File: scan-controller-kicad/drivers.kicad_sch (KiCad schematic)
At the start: 45 parts, among them CN4 Fan, CN5 Motor, CN6 Lamp, Q6 SS8050, Q7 IRF7470, U5 DRV8871DDA, U6 78L05, U7 XL4015, U8 TL431, U9 LM358

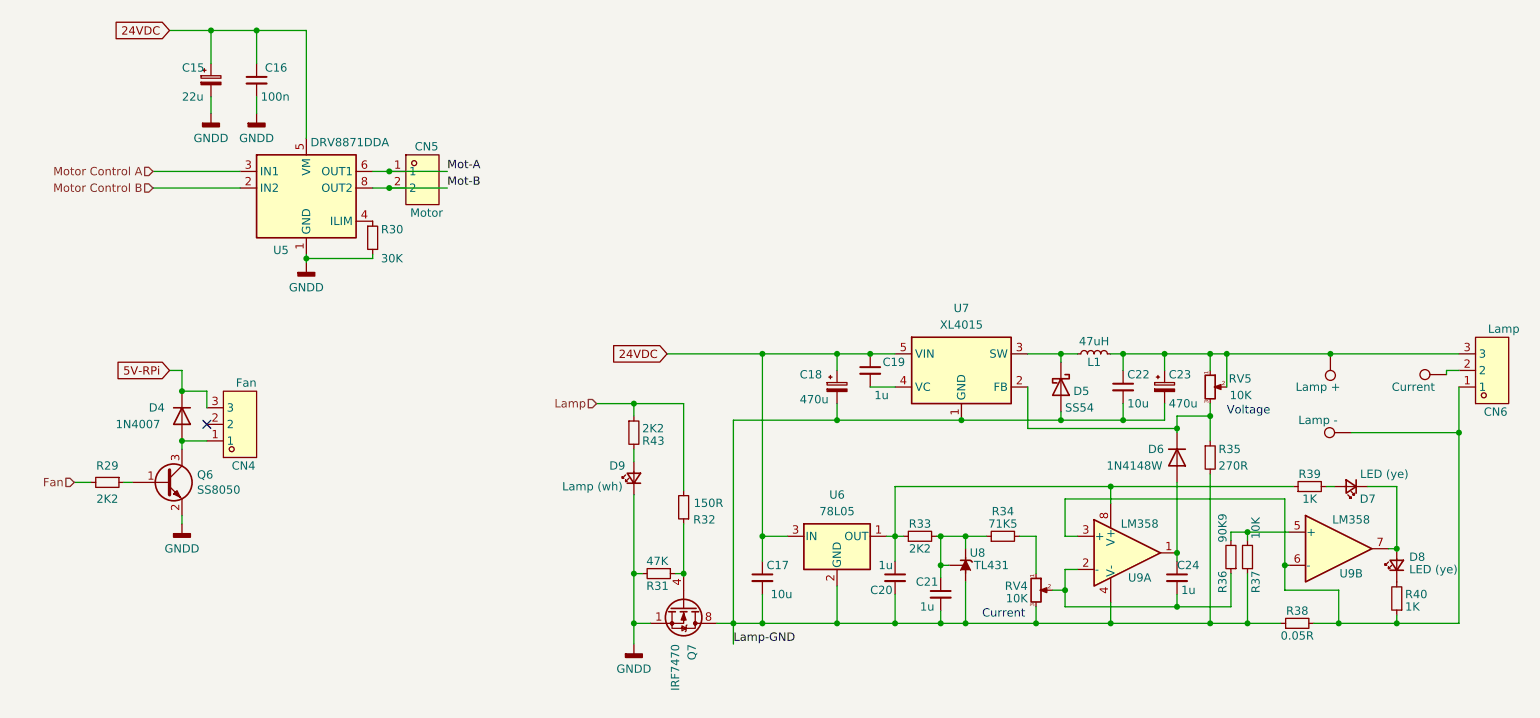
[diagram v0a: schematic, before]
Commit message: Lamp Driver final, but now off grid :-?
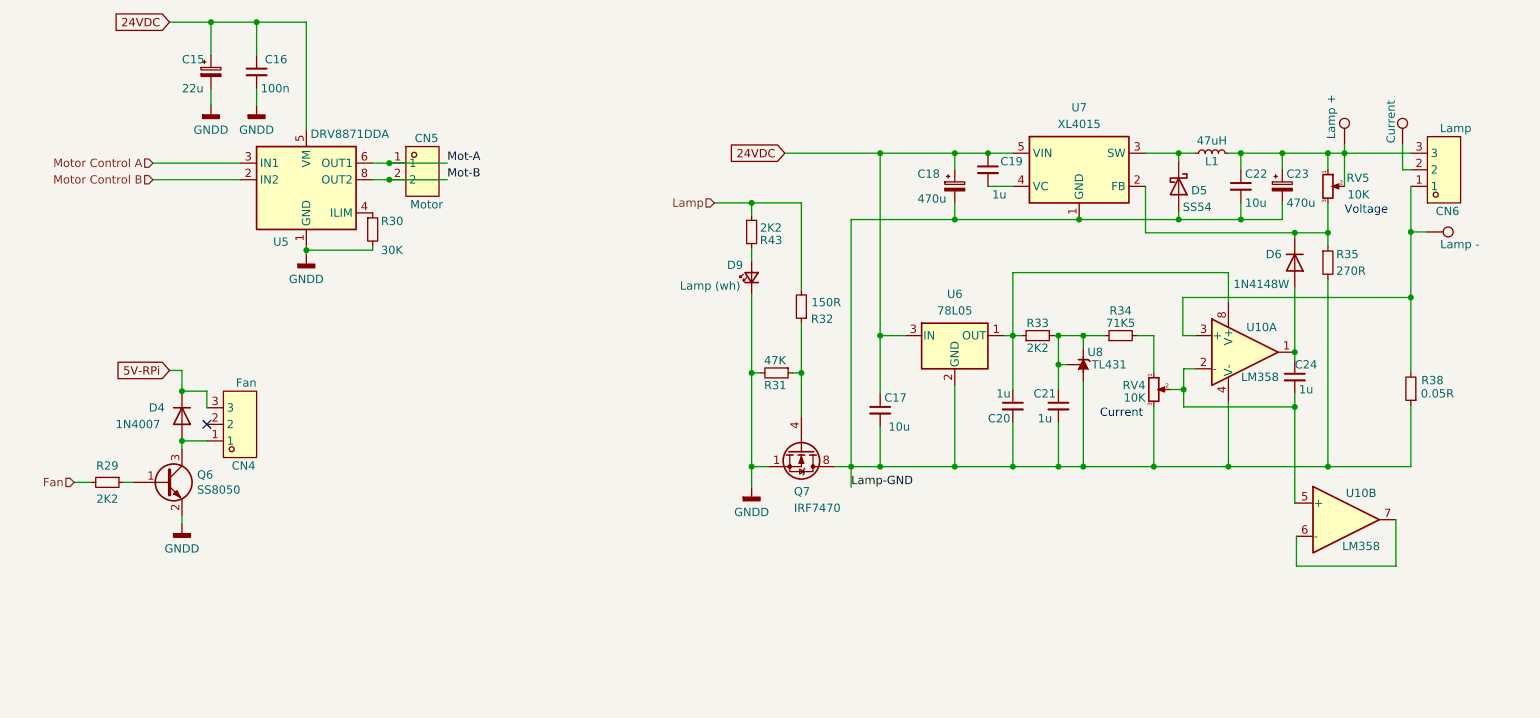
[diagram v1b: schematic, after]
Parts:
- removed D7, D8: LED (ye), LED_SMD:LED_0805_2012Metric, symbol Device:LED_Small
- removed R36: 90K9, Resistor_SMD:R_0805_2012Metric, symbol Device:R_Small
- removed R37: 10K, Resistor_SMD:R_0805_2012Metric, symbol Device:R_Small
- removed R39, R40: 1K, Resistor_SMD:R_0805_2012Metric, symbol Device:R_Small
- removed U9: LM358, Package_SO:SOIC-8_3.9x4.9mm_P1.27mm, symbol Amplifier_Operational:LM358
- added U10: LM358, Package_SO:SOIC-8_3.9x4.9mm_P1.27mm, symbol Amplifier_Operational:LM358
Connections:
- net Lamp-GND: now also U10.4 (V-)
- net at C20.1, R33.1, U6.1 (OUT): now also U10.8 (V+)
- net at C24.2, RV4.2: now also U10.2 (-), U10.5 (+)
- net at C24.1, D6.2 (A): now also U10.1
- net at CN6.1, R38.2, TP15.1: now also U10.3 (+)
- new net: U10.6 (-), U10.7
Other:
- moved on the sheet: C15, C16, C17, C18, C19, C20, C21, C22, C23, C24, CN5, CN6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

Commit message: Fixing the Lamp Driver Grid
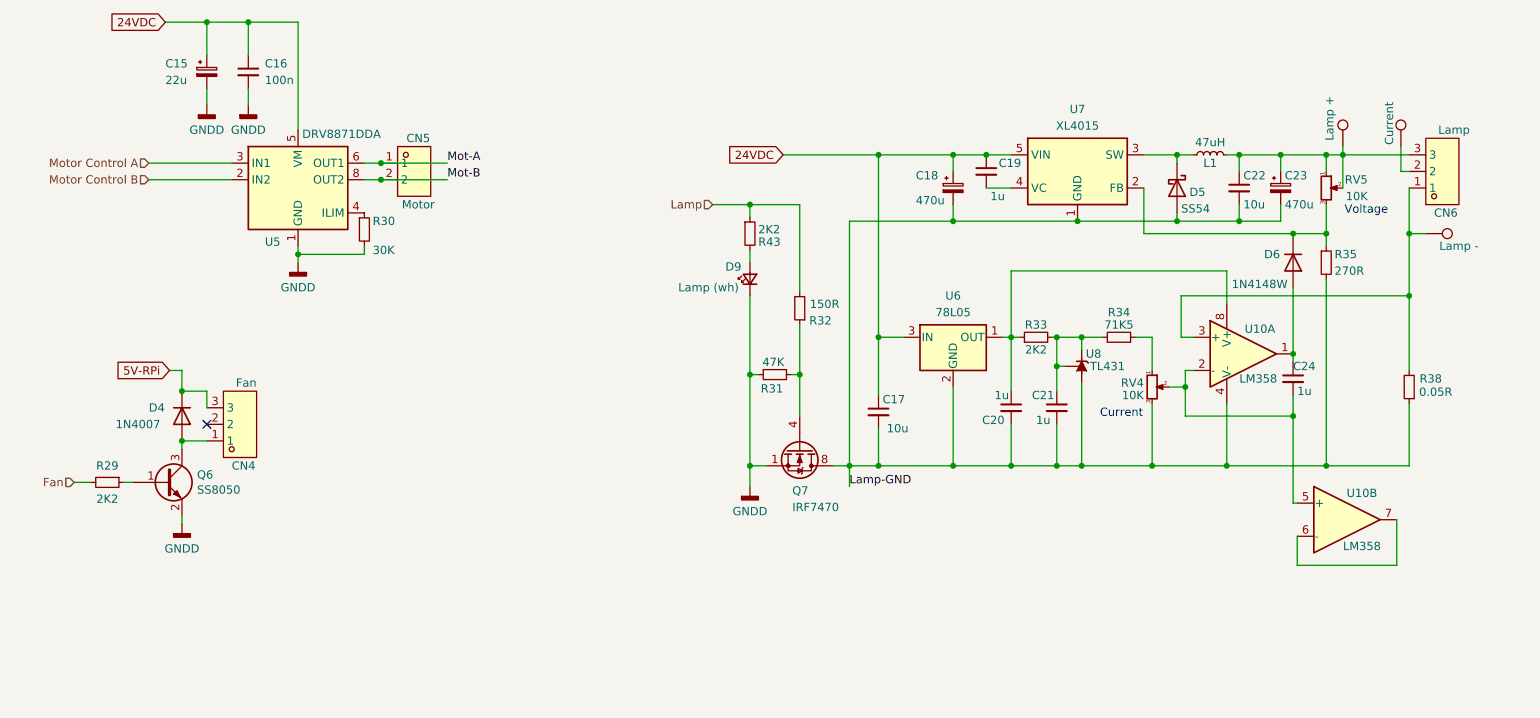
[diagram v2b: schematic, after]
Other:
- moved on the sheet: C15, C16, CN5, R30, U5
